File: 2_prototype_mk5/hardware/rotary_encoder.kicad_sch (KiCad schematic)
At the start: 2 parts, among them J7 Conn_01x05, SW3 PEC12R-2120F-S0012

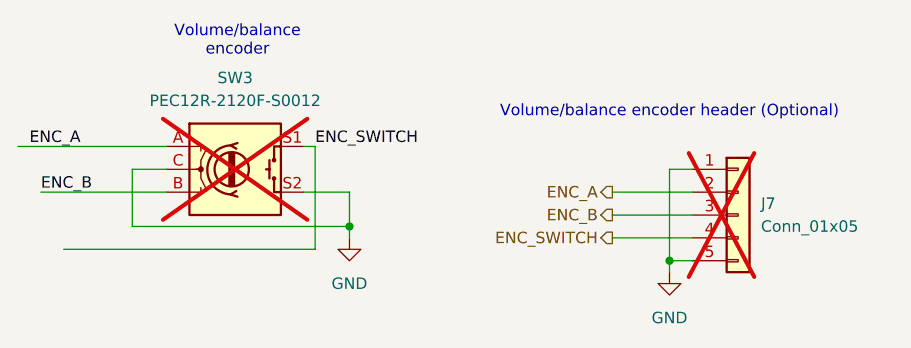
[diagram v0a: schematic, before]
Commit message: MK5 revision 2 hardware updates and ISA adapter revisions
Ignore VSCode local-history artifacts going forward.

Co-Authored-By: Claude Sonnet 5 <noreply@anthropic.com>
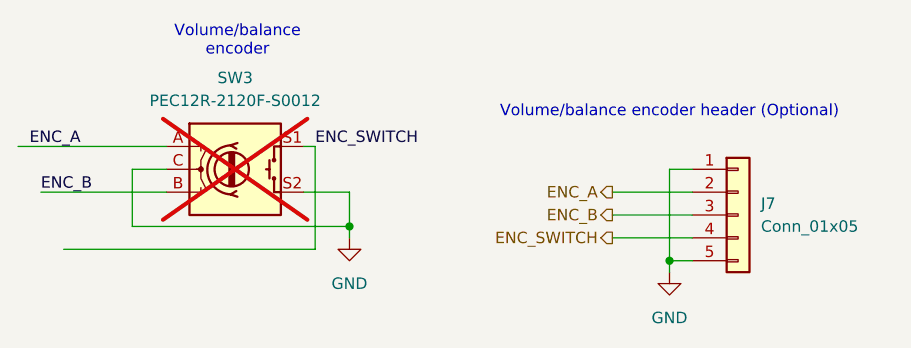
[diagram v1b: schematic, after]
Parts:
- J7: now fitted; now in the parts list
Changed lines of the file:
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@@
 		(body_style 1)
 		(exclude_from_sim no)
-		(in_bom no)
+		(in_bom yes)
 		(on_board yes)
 		(in_pos_files yes)
-		(dnp yes)
+		(dnp no)
 		(fields_autoplaced yes)
 		(property "Reference" "J7"
